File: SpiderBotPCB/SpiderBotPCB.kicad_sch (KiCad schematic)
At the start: 12 parts, among them U1 STM32L412KBT6, U2 L7986A

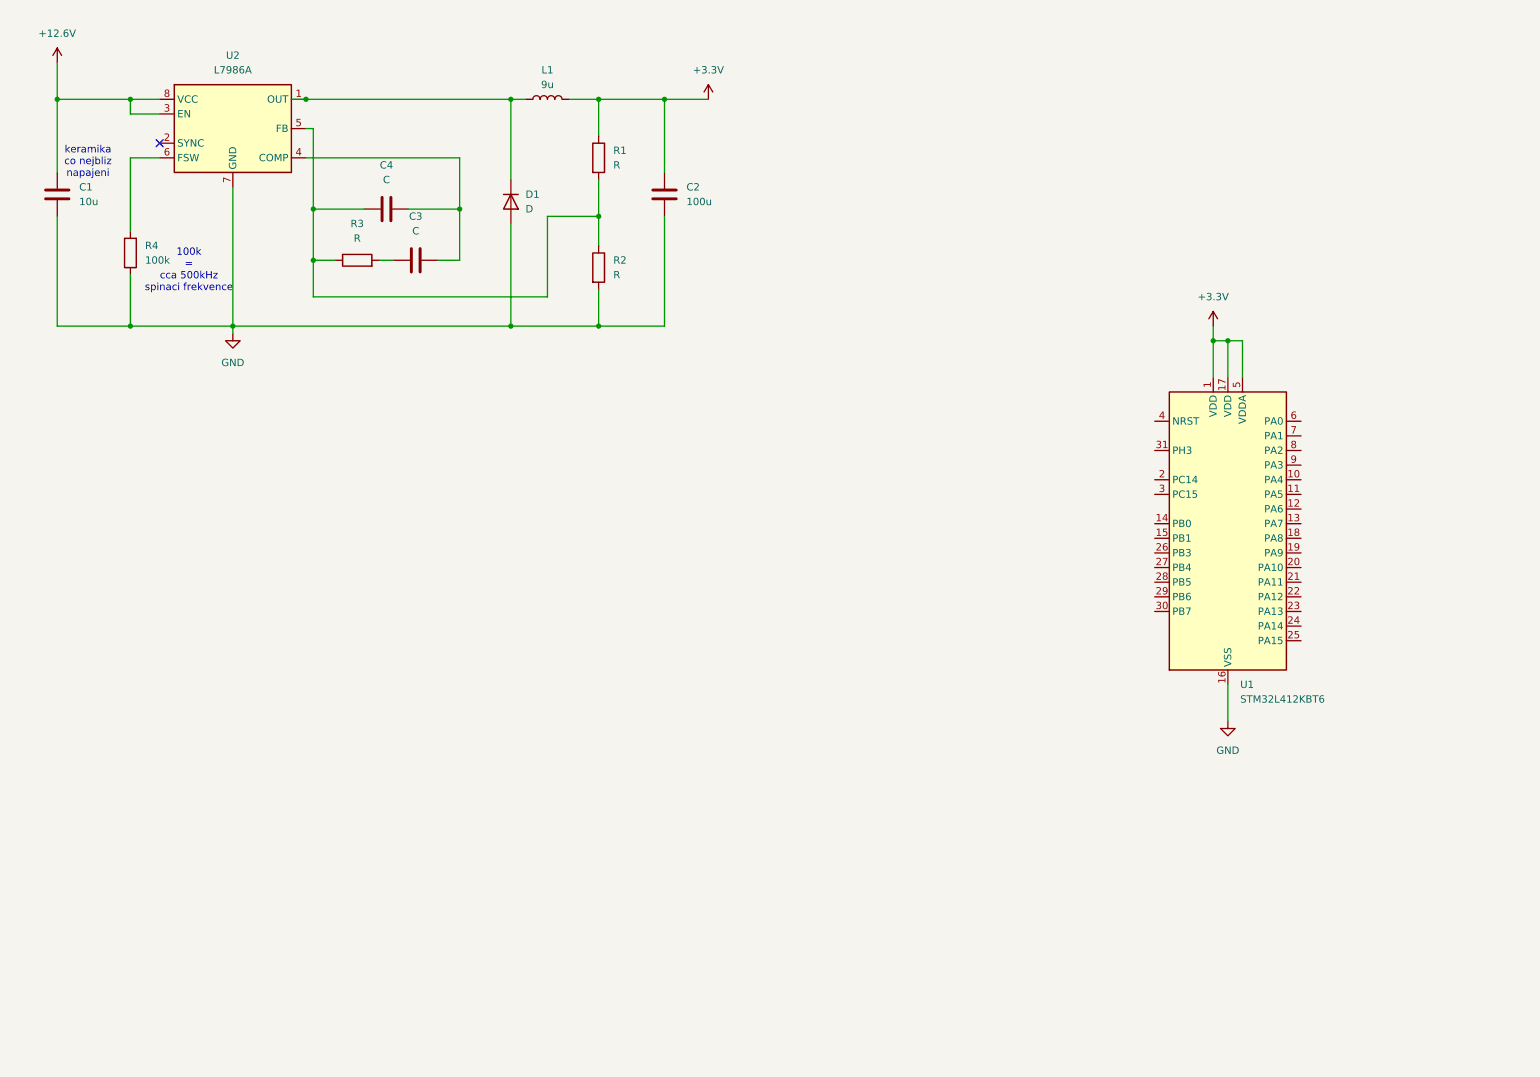
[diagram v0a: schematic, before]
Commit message: add stuff
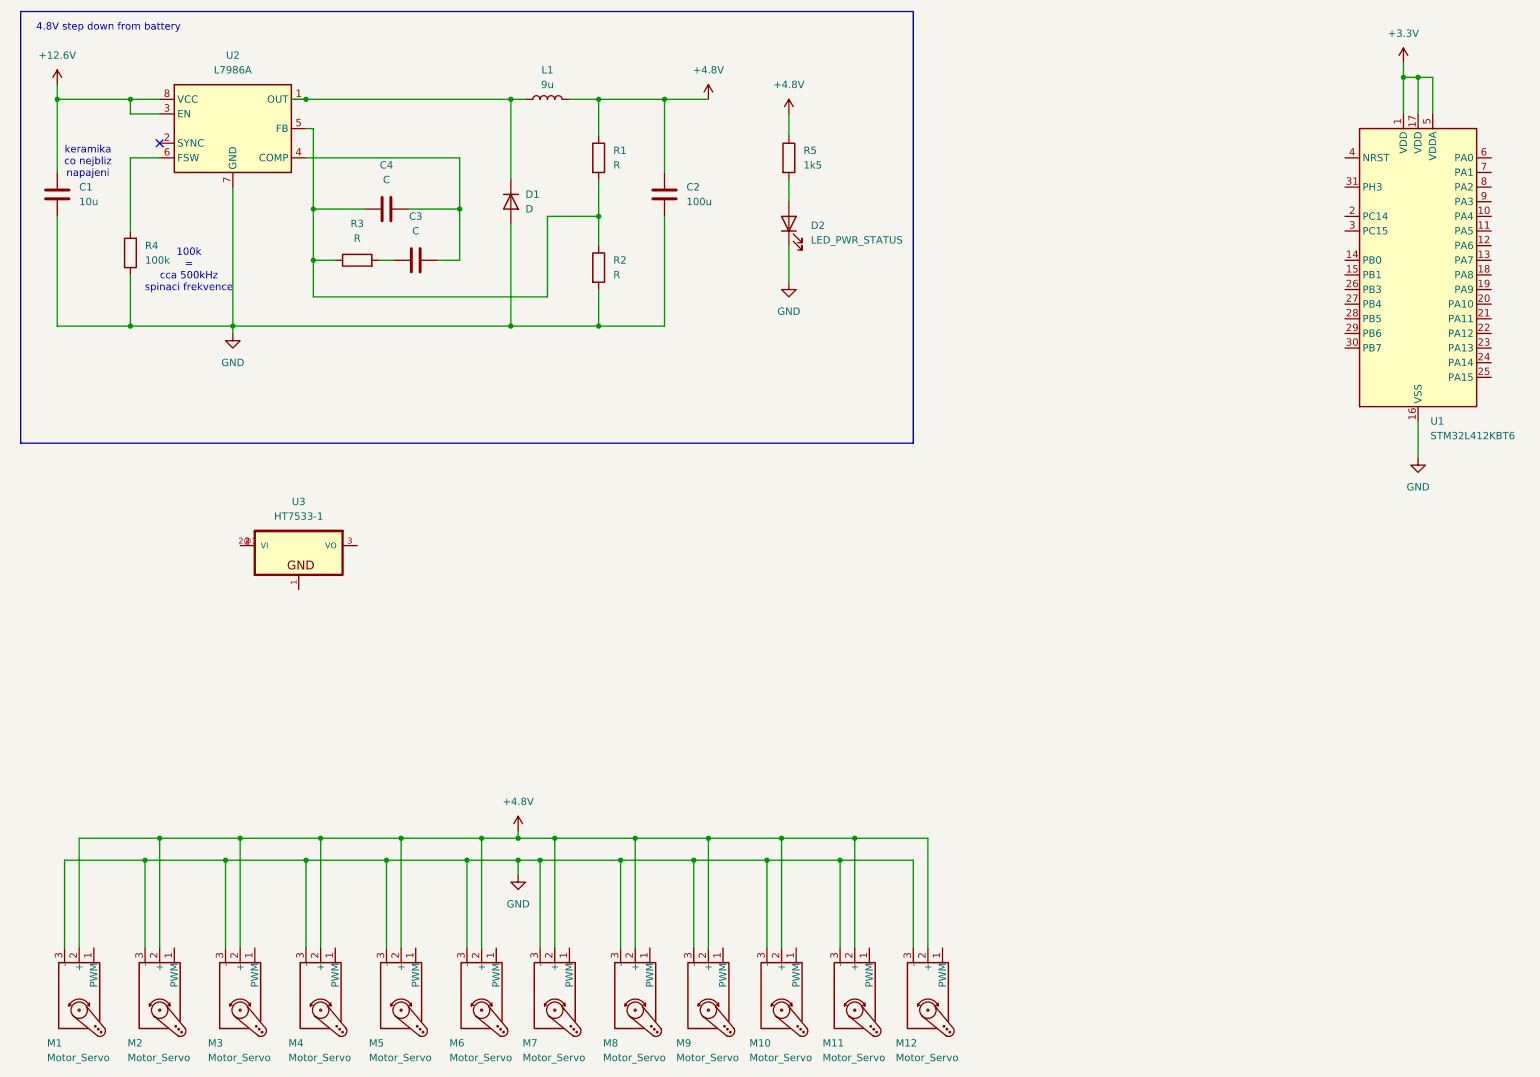
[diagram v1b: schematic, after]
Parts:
- added D2: LED_PWR_STATUS, symbol Device:LED
- added M1, M10, M11, M12, M2, M3, M4, M5, M6, M7, M8, M9: Motor_Servo, symbol Motor:Motor_Servo
- added R5: 1k5, symbol Device:R
- added U3: HT7533-1, HT7533-1:SOT89, symbol HT7533:HT7533-1
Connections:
- net +3.3V: no longer C2.2, L1.2, R1.1
- net GND: now also D2.1 (K), M1.3 (-), M10.3 (-), M11.3 (-), M12.3 (-), M2.3 (-), M3.3 (-), M4.3 (-), M5.3 (-), M6.3 (-), M7.3 (-), M8.3 (-), M9.3 (-)
- new net: U3.2 (VI), U3.2@1 (VI)
- new net: D2.2 (A), R5.2
- new net +4.8V: C2.2, L1.2, M1.2 (+), M10.2 (+), M11.2 (+), M12.2 (+), M2.2 (+), M3.2 (+), M4.2 (+), M5.2 (+), M6.2 (+), M7.2 (+), M8.2 (+), M9.2 (+), R1.1, R5.1
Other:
- note added: "4.8V step down from battery"
- moved on the sheet: U1
